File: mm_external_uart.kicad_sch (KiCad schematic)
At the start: 1 part, among them J6 Conn_01x04_Pin

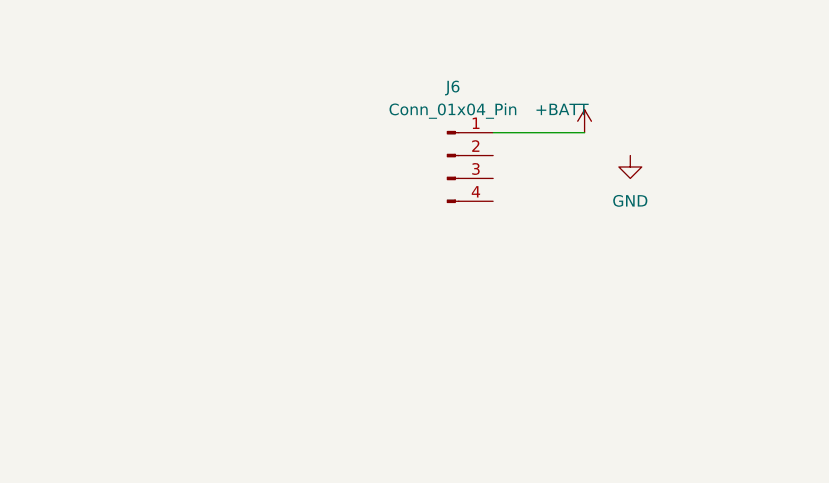
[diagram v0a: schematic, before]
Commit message: TP3
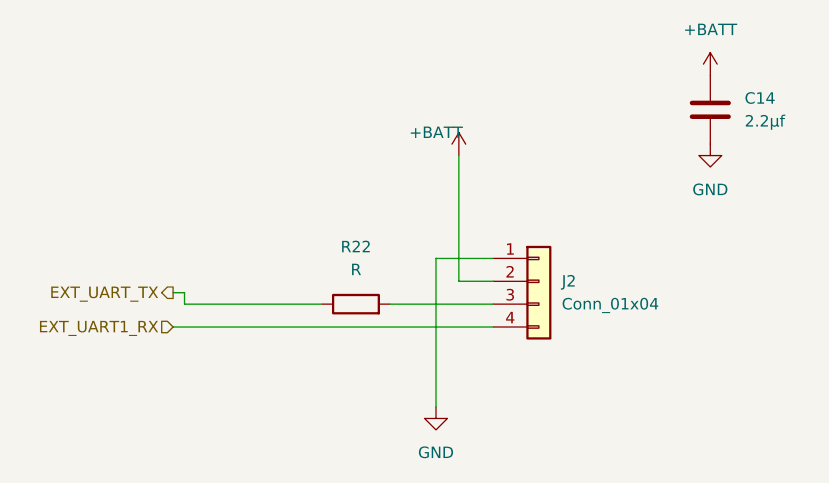
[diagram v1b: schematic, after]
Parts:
- removed J6: Conn_01x04_Pin, symbol Connector:Conn_01x04_Pin
- added C14: 2.2µf, Capacitor_SMD:C_0603_1608Metric, symbol Device:C
- added J2: Conn_01x04, Connector_PinHeader_2.54mm:PinHeader_1x04_P2.54mm_Vertical, symbol Connector_Generic:Conn_01x04
- added R22: R, Resistor_SMD:R_0603_1608Metric, symbol Device:R
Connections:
- net +BATT: now also C14.1, J2.2 (Pin_2)
- net GND: now also C14.2, J2.1 (Pin_1)
- new net: J2.3 (Pin_3), R22.2
- new net EXT_UART1_RX: J2.4 (Pin_4)
- new net EXT_UART_TX: R22.1
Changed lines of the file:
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@@
 (kicad_sch (version 20230121) (generator eeschema)
   (paper "A4")
-  (wire (pts (xy 142.24 93.98) (xy 152.4 93.98))
+  (wire (pts (xy 135.89 124.46) (xy 135.89 107.95))
     (stroke (width 0) (type default))
   )
-  (symbol (lib_id "power:GND") (at 157.48 96.52 0) (unit 1)
+  (wire (pts (xy 123.19 113.03) (xy 107.95 113.03))
+    (stroke (width 0) (type default))
+  )
+  (wire (pts (xy 135.89 107.95) (xy 142.24 107.95))
+    (stroke (width 0) (type default))
+  )
+  (wire (pts (xy 138.43 110.49) (xy 142.24 110.49))
+    (stroke (width 0) (type default))
+  )
+  (wire (pts (xy 107.95 111.76) (xy 106.68 111.76))
+    (stroke (width 0) (type default))
+  )
+  (wire (pts (xy 106.68 115.57) (xy 142.24 115.57))
+    (stroke (width 0) (type default))
+  )
+  (wire (pts (xy 138.43 96.52) (xy 138.43 110.49))
+    (stroke (width 0) (type default))
+  )
+  (wire (pts (xy 107.95 113.03) (xy 107.95 111.76))
+    (stroke (width 0) (type default))
+  )
+  (wire (pts (xy 130.81 113.03) (xy 142.24 113.03))
+    (stroke (width 0) (type default))
+  )
+  (hierarchical_label "EXT_UART_TX" (shape output) (at 106.68 111.76 180) (fields_autoplaced)
+    (effects (font (size 1.27 1.27)) (justify right))
+  )
+  (hierarchical_label "EXT_UART1_RX" (shape input) (at 106.68 115.57 180) (fields_autoplaced)
+    (effects (font (size 1.27 1.27)) (justify right))
+  )
+  (symbol (lib_id "power:GND") (at 135.89 124.46 0) (unit 1)
     (in_bom yes) (on_board yes) (dnp no) (fields_autoplaced)
-    (property "Reference" "#PWR016" (at 157.48 102.87 0)
+    (property "Reference" "#PWR030" (at 135.89 130.81 0)
       (effects (font (size 1.27 1.27)) hide)
     )
-    (property "Value" "GND" (at 157.48 101.6 0)
+    (property "Value" "GND" (at 135.89 129.54 0)
       (effects (font (size 1.27 1.27)))
     )
-    (property "Footprint" "" (at 157.48 96.52 0)
+    (property "Footprint" "" (at 135.89 124.46 0)
       (effects (font (size 1.27 1.27)) hide)
     )
-    (property "Datasheet" "" (at 157.48 96.52 0)
+    (property "Datasheet" "" (at 135.89 124.46 0)
+      (effects (font (size 1.27 1.27)) hide)
+    )
+    (pin "1")
+    (instances
+      (project "minimouse"
+        (path "/d8fa4cba-2469-4231-847f-065b6b829f44/d17bb1c7-f68a-465e-9a17-5858ef86fc30"
+          (reference "#PWR030") (unit 1)
+        )
+      )
+    )
+  )
+  (symbol (lib_id "power:+BATT") (at 166.37 87.63 0) (unit 1)
+    (in_bom yes) (on_board yes) (dnp no) (fields_autoplaced)
+    (property "Reference" "#PWR029" (at 166.37 91.44 0)
+      (effects (font (size 1.27 1.27)) hide)
+    )
+    (property "Value" "+BATT" (at 166.37 82.55 0)
+      (effects (font (size 1.27 1.27)))
+    )
+    (property "Footprint" "" (at 166.37 87.63 0)
+      (effects (font (size 1.27 1.27)) hide)
+    )
+    (property "Datasheet" "" (at 166.37 87.63 0)
+      (effects (font (size 1.27 1.27)) hide)
+    )
+    (pin "1")
+    (instances
+      (project "minimouse"
+        (path "/d8fa4cba-2469-4231-847f-065b6b829f44/d17bb1c7-f68a-465e-9a17-5858ef86fc30"
+          (reference "#PWR029") (unit 1)
+        )
+      )
+    )
+  )
+  (symbol (lib_id "power:GND") (at 166.37 95.25 0) (unit 1)
+    (in_bom yes) (on_board yes) (dnp no) (fields_autoplaced)
+    (property "Reference" "#PWR016" (at 166.37 101.6 0)
+      (effects (font (size 1.27 1.27)) hide)
+    )
+    (property "Value" "GND" (at 166.37 100.33 0)
+      (effects (font (size 1.27 1.27)))
+    )
+    (property "Footprint" "" (at 166.37 95.25 0)
+      (effects (font (size 1.27 1.27)) hide)
+    )
+    (property "Datasheet" "" (at 166.37 95.25 0)
       (effects (font (size 1.27 1.27)) hide)
     )
@@
     )
   )
-  (symbol (lib_id "power:+BATT") (at 152.4 93.98 0) (unit 1)
-    (in_bom yes) (on_board yes) (dnp no)
-    (property "Reference" "#PWR036" (at 152.4 97.79 0)
+  (symbol (lib_id "Device:C") (at 166.37 91.44 0) (unit 1)
+    (in_bom yes) (on_board yes) (dnp no) (fields_autoplaced)
+    (property "Reference" "C14" (at 170.18 90.17 0)
+      (effects (font (size 1.27 1.27)) (justify left))
+    )
+    (property "Value" "2.2µf" (at 170.18 92.71 0)
+      (effects (font (size 1.27 1.27)) (justify left))
+    )
+    (property "Footprint" "Capacitor_SMD:C_0603_1608Metric" (at 167.3352 95.25 0)
       (effects (font (size 1.27 1.27)) hide)
     )
-    (property "Value" "+BATT" (at 149.86 91.44 0)
+    (property "Datasheet" "~" (at 166.37 91.44 0)
+      (effects (font (size 1.27 1.27)) hide)
+    )
+    (pin "1")
+    (pin "2")
+    (instances
+      (project "minimouse"
+        (path "/d8fa4cba-2469-4231-847f-065b6b829f44/d17bb1c7-f68a-465e-9a17-5858ef86fc30"
+          (reference "C14") (unit 1)
+        )
+      )
+    )
+  )
+  (symbol (lib_id "power:+BATT") (at 138.43 96.52 0) (unit 1)
+    (in_bom yes) (on_board yes) (dnp no)
+    (property "Reference" "#PWR015" (at 138.43 100.33 0)
+      (effects (font (size 1.27 1.27)) hide)
+    )
+    (property "Value" "+BATT" (at 135.89 93.98 0)
       (effects (font (size 1.27 1.27)))
     )
-    (property "Footprint" "" (at 152.4 93.98 0)
+    (property "Footprint" "" (at 138.43 96.52 0)
       (effects (font (size 1.27 1.27)) hide)
     )
-    (property "Datasheet" "" (at 152.4 93.98 0)
+    (property "Datasheet" "" (at 138.43 96.52 0)
       (effects (font (size 1.27 1.27)) hide)
     )
@@
     (instances
       (project "minimouse"
-        (path "/d8fa4cba-2469-4231-847f-065b6b829f44/3f9b0845-5778-418c-a7a8-03da2392145e"
-          (reference "#PWR036") (unit 1)
-        )
         (path "/d8fa4cba-2469-4231-847f-065b6b829f44/d17bb1c7-f68a-465e-9a17-5858ef86fc30"
           (reference "#PWR015") (unit 1)
@@
     )
   )
-  (symbol (lib_id "Connector:Conn_01x04_Pin") (at 137.16 96.52 0) (unit 1)
+  (symbol (lib_id "Connector_Generic:Conn_01x04") (at 147.32 110.49 0) (unit 1)
     (in_bom yes) (on_board yes) (dnp no) (fields_autoplaced)
-    (property "Reference" "J6" (at 137.795 88.9 0)
-      (effects (font (size 1.27 1.27)))
+    (property "Reference" "J2" (at 149.86 110.49 0)
+      (effects (font (size 1.27 1.27)) (justify left))
     )
-    (property "Value" "Conn_01x04_Pin" (at 137.795 91.44 0)
-      (effects (font (size 1.27 1.27)))
+    (property "Value" "Conn_01x04" (at 149.86 113.03 0)
+      (effects (font (size 1.27 1.27)) (justify left))
     )
-    (property "Footprint" "" (at 137.16 96.52 0)
+    (property "Footprint" "Connector_PinHeader_2.54mm:PinHeader_1x04_P2.54mm_Vertical" (at 147.32 110.49 0)
       (effects (font (size 1.27 1.27)) hide)
     )
-    (property "Datasheet" "~" (at 137.16 96.52 0)
+    (property "Datasheet" "~" (at 147.32 110.49 0)
       (effects (font (size 1.27 1.27)) hide)
     )
+    (pin "3")
+    (pin "4")
     (pin "1")
     (pin "2")
-    (pin "4")
-    (pin "3")
     (instances
       (project "minimouse"
         (path "/d8fa4cba-2469-4231-847f-065b6b829f44/d17bb1c7-f68a-465e-9a17-5858ef86fc30"
-          (reference "J6") (unit 1)
+          (reference "J2") (unit 1)
         )
       )
+    )
+  )
+  (symbol (lib_id "Device:R") (at 127 113.03 90) (unit 1)
+    (in_bom yes) (on_board yes) (dnp no) (fields_autoplaced)
+    (property "Reference" "R22" (at 127 106.68 90)
+      (effects (font (size 1.27 1.27)))
+    )
+    (property "Value" "R" (at 127 109.22 90)
+      (effects (font (size 1.27 1.27)))
+    )
+    (property "Footprint" "Resistor_SMD:R_0603_1608Metric" (at 127 114.808 90)
+      (effects (font (size 1.27 1.27)) hide)
+    )
+    (property "Datasheet" "~" (at 127 113.03 0)
+      (effects (font (size 1.27 1.27)) hide)
+    )
+    (pin "2")
+    (pin "1")
+    (instances
+      (project "minimouse"
+        (path "/d8fa4cba-2469-4231-847f-065b6b829f44/d17bb1c7-f68a-465e-9a17-5858ef86fc30"
+          (reference "R22") (unit 1)
+        )
+      )
